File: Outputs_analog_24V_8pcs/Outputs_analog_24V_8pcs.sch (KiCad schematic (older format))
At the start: 10 parts, among them J1 Screw_Terminal_01x02, J2 Screw_Terminal_01x02, J3 Screw_Terminal_01x06, U1 74HC595

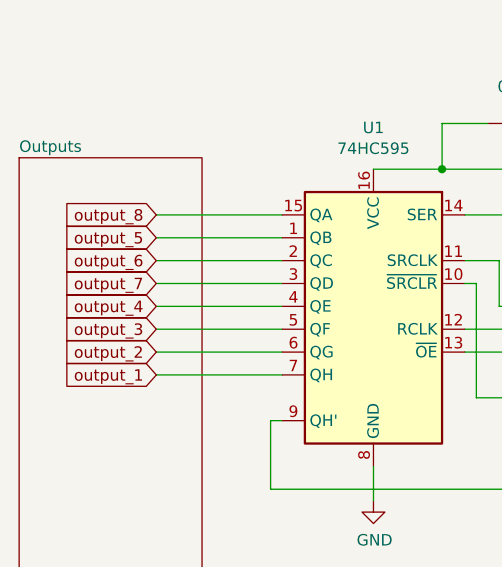
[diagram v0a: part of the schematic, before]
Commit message: Update pcb
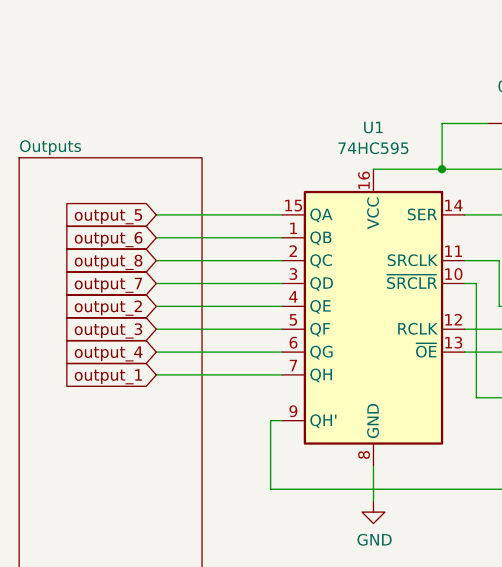
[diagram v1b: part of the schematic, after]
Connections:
- net output_2: now also U1.4 (QE); no longer U1.6 (QG)
- net output_4: now also U1.6 (QG); no longer U1.4 (QE)
- net output_5: now also U1.15 (QA); no longer U1.1 (QB)
- net output_6: now also U1.1 (QB); no longer U1.2 (QC)
- net output_8: now also U1.2 (QC); no longer U1.15 (QA)
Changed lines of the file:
@@
 EESchema Schematic File Version 4
-LIBS:Outputs_analog_24V_8pcs-cache
-EELAYER 26 0
+EELAYER 30 0
 EELAYER END
 $Descr A4 11693 8268
@@
 Text GLabel 1600 4300 0    50   Input ~ 0
 output_1
-Text GLabel 1600 4200 0    50   Input ~ 0
+Text GLabel 1600 4000 0    50   Input ~ 0
 output_2
 Text GLabel 1600 4100 0    50   Input ~ 0
 output_3
-Text GLabel 1600 4000 0    50   Input ~ 0
+Text GLabel 1600 4200 0    50   Input ~ 0
 output_4
+Text GLabel 1600 3600 0    50   Input ~ 0
+output_5
 Text GLabel 1600 3700 0    50   Input ~ 0
-output_5
-Text GLabel 1600 3800 0    50   Input ~ 0
 output_6
 Text GLabel 1600 3900 0    50   Input ~ 0
 output_7
-Text GLabel 1600 3600 0    50   Input ~ 0
+Text GLabel 1600 3800 0    50   Input ~ 0
 output_8
 $Comp
@@
 	1600 4300 2150 4300
 Wire Wire Line
-	1600 4200 2150 4200
-Wire Wire Line
 	1600 4100 2150 4100
-Wire Wire Line
-	1600 4000 2150 4000
-Wire Wire Line
-	1600 3600 2150 3600
-Wire Wire Line
-	1600 3900 2150 3900
-Wire Wire Line
-	1600 3700 2150 3700
 Wire Wire Line
 	1600 3800 2150 3800
@@
 Wire Wire Line
 	3400 4200 3550 4200
+Wire Wire Line
+	1600 4200 2150 4200
+Wire Wire Line
+	1600 4000 2150 4000
+Wire Wire Line
+	1600 3700 2150 3700
+Wire Wire Line
+	1600 3900 2150 3900
+Wire Wire Line
+	1600 3600 2150 3600
 $EndSCHEMATC
